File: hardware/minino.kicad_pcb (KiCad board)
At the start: 2 copper layers, 45 x 68 mm, 58 parts, among them J1 OLED, J2 GPS, J3 Battery, P1 USB_C_Plug_USB2.0, Q1 DMG3415U-7, Q2 MMBT2222A, SW1 ON, SW2 RIGHT, SW3 LEFT, SW4 DOWN, SW5 UP, SW6 OK, SW7 RESET, SW8 GPIO, U1 ESP32-S3-WROOM-1U-N16, U2 MCP73831-3-OT, U3 AP2112K-3.3

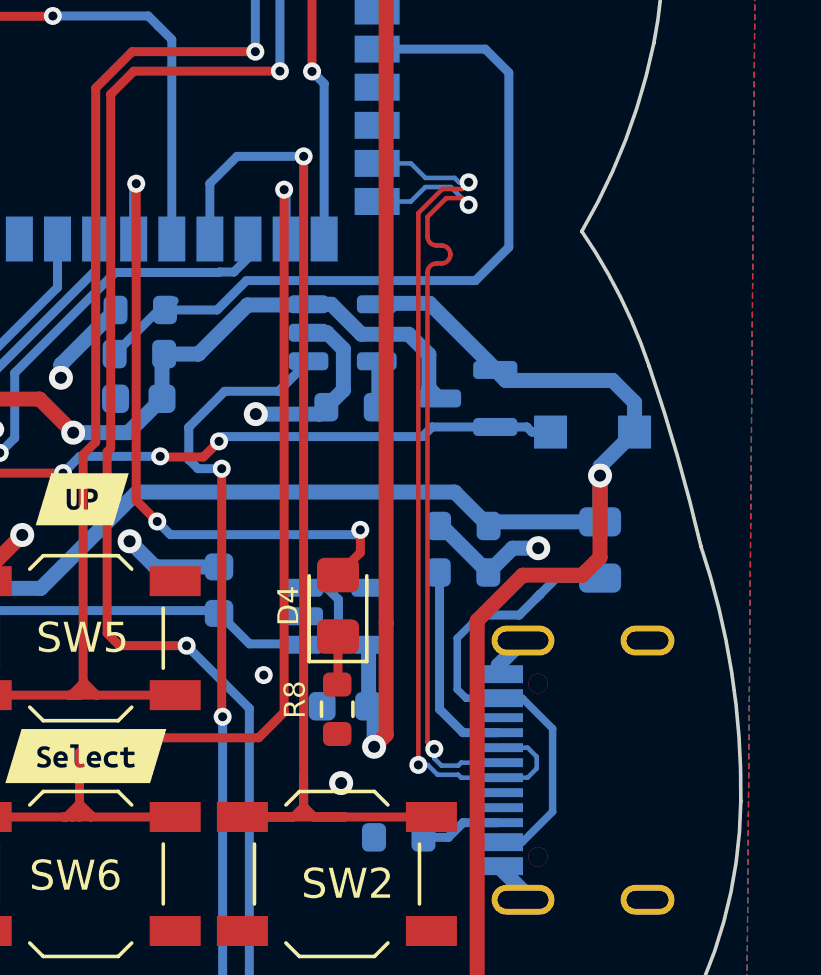
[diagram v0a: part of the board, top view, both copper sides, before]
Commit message: Add_example
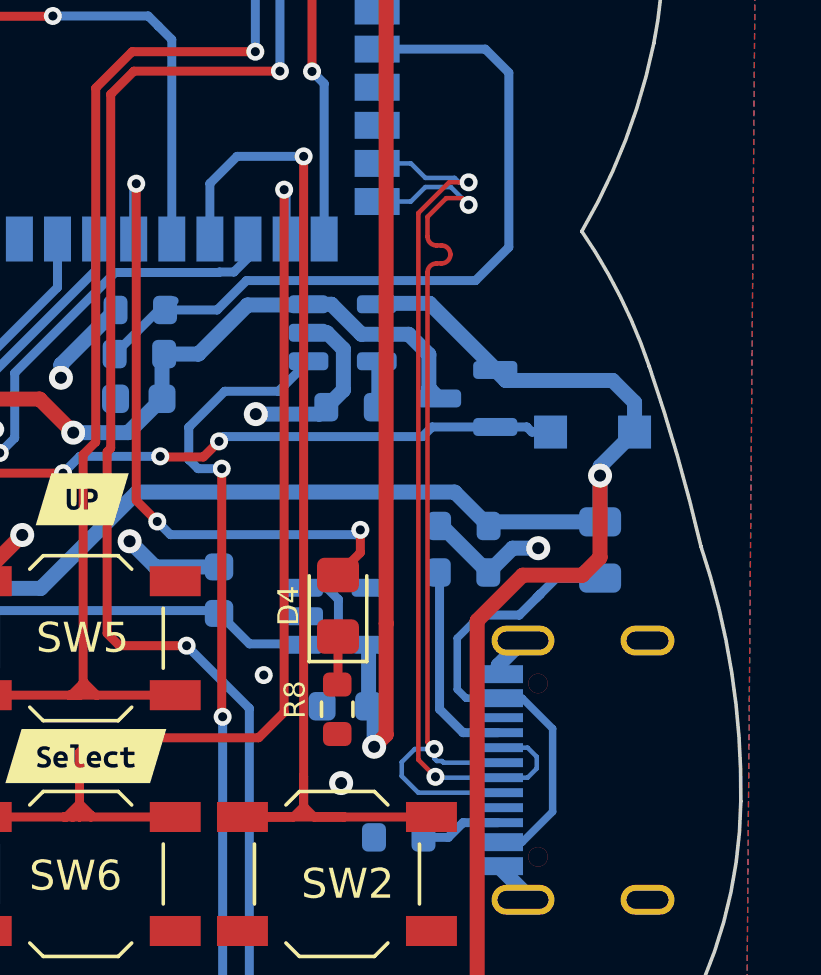
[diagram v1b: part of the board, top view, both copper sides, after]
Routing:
- net /D+: track 26.6 -> 31.7 mm
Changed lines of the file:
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@@
   (segment (start 198.585 76.82) (end 198.61 76.845) (width 0.3) (layer "B.Cu") (net 13))
   (segment (start 199.3925 82.16) (end 200.5675 82.16) (width 0.3) (layer "B.Cu") (net 13))
-  (segment (start 197.903986 64.840486) (end 198.706873 64.037599) (width 0.1524) (layer "F.Cu") (net 14))
-  (segment (start 197.903986 83.236014) (end 197.903986 64.840486) (width 0.1524) (layer "F.Cu") (net 14))
-  (segment (start 199.356201 64.037599) (end 199.58 63.8138) (width 0.1524) (layer "F.Cu") (net 14))
-  (segment (start 198.706873 64.037599) (end 199.356201 64.037599) (width 0.1524) (layer "F.Cu") (net 14))
+  (segment (start 198.930672 63.8138) (end 197.903986 64.840486) (width 0.1524) (layer "F.Cu") (net 14))
+  (segment (start 197.903986 83.062879) (end 198.473007 83.6319) (width 0.1524) (layer "F.Cu") (net 14))
+  (segment (start 199.58 63.8138) (end 198.930672 63.8138) (width 0.1524) (layer "F.Cu") (net 14))
+  (segment (start 197.903986 64.840486) (end 197.903986 83.062879) (width 0.1524) (layer "F.Cu") (net 14))
   (via (at 199.58 63.8138) (size 0.6) (drill 0.3) (layers "F.Cu" "B.Cu") (net 14))
-  (via (at 197.903986 83.236014) (size 0.6) (drill 0.3) (layers "F.Cu" "B.Cu") (net 14))
+  (via (at 198.473007 83.6319) (size 0.6) (drill 0.3) (layers "F.Cu" "B.Cu") (net 14))
   (segment (start 198.137601 63.6676) (end 197.655001 63.185) (width 0.1524) (layer "B.Cu") (net 14))
-  (segment (start 198.546873 83.5624) (end 198.220487 83.236014) (width 0.1524) (layer "B.Cu") (net 14))
-  (segment (start 199.232399 83.5624) (end 198.546873 83.5624) (width 0.1524) (layer "B.Cu") (net 14))
-  (segment (start 199.329999 83.66) (end 199.232399 83.5624) (width 0.1524) (layer "B.Cu") (net 14))
   (segment (start 201.85 83.3549) (end 201.85 82.9651) (width 0.1524) (layer "B.Cu") (net 14))
+  (segment (start 200.5675 83.66) (end 198.501107 83.66) (width 0.1524) (layer "B.Cu") (net 14))
+  (segment (start 198.501107 83.66) (end 198.473007 83.6319) (width 0.1524) (layer "B.Cu") (net 14))
   (segment (start 201.5449 82.66) (end 200.5675 82.66) (width 0.1524) (layer "B.Cu") (net 14))
   (segment (start 199.112453 63.6676) (end 198.137601 63.6676) (width 0.1524) (layer "B.Cu") (net 14))
@@
   (segment (start 201.85 82.9651) (end 201.5449 82.66) (width 0.1524) (layer "B.Cu") (net 14))
   (segment (start 200.5675 83.66) (end 201.5449 83.66) (width 0.1524) (layer "B.Cu") (net 14))
-  (segment (start 200.5675 83.66) (end 199.329999 83.66) (width 0.1524) (layer "B.Cu") (net 14))
   (segment (start 199.58 63.8138) (end 199.258653 63.8138) (width 0.1524) (layer "B.Cu") (net 14))
   (segment (start 201.5449 83.66) (end 201.85 83.3549) (width 0.1524) (layer "B.Cu") (net 14))
   (segment (start 197.655001 63.185) (end 196.53 63.185) (width 0.1524) (layer "B.Cu") (net 14))
-  (segment (start 198.220487 83.236014) (end 197.903986 83.236014) (width 0.1524) (layer "B.Cu") (net 14))
   (segment (start 198.833127 64.342401) (end 198.208786 64.966742) (width 0.1524) (layer "F.Cu") (net 15))
   (segment (start 198.208786 66.818786) (end 198.208786 66.868786) (width 0.1524) (layer "F.Cu") (net 15))
@@
   (arc (start 198.508786 66.518786) (mid 198.296654 66.606654) (end 198.208786 66.818786) (width 0.1524) (layer "F.Cu") (net 15))
   (arc (start 198.6713 65.918786) (mid 198.883432 66.006654) (end 198.9713 66.218786) (width 0.1524) (layer "F.Cu") (net 15))
+  (segment (start 197.35 83.61) (end 197.35 83.14) (width 0.1524) (layer "B.Cu") (net 15))
   (segment (start 197.655001 64.455) (end 196.53 64.455) (width 0.1524) (layer "B.Cu") (net 15))
-  (segment (start 199.232399 83.2576) (end 198.673127 83.2576) (width 0.1524) (layer "B.Cu") (net 15))
-  (segment (start 198.673127 83.2576) (end 198.436014 83.020487) (width 0.1524) (layer "B.Cu") (net 15))
-  (segment (start 199.329999 83.16) (end 199.232399 83.2576) (width 0.1524) (layer "B.Cu") (net 15))
-  (segment (start 200.5675 83.16) (end 199.329999 83.16) (width 0.1524) (layer "B.Cu") (net 15))
+  (segment (start 200.5675 83.16) (end 198.747264 83.16) (width 0.1524) (layer "B.Cu") (net 15))
+  (segment (start 198.691754 83.10449) (end 198.520017 83.10449) (width 0.1524) (layer "B.Cu") (net 15))
+  (segment (start 198.747264 83.16) (end 198.691754 83.10449) (width 0.1524) (layer "B.Cu") (net 15))
+  (segment (start 200.5675 84.16) (end 197.9 84.16) (width 0.1524) (layer "B.Cu") (net 15))
+  (segment (start 197.786014 82.703986) (end 198.436014 82.703986) (width 0.1524) (layer "B.Cu") (net 15))
+  (segment (start 197.35 83.14) (end 197.786014 82.703986) (width 0.1524) (layer "B.Cu") (net 15))
   (segment (start 198.9862 63.9724) (end 198.137601 63.9724) (width 0.1524) (layer "B.Cu") (net 15))
   (segment (start 199.58 64.5662) (end 198.9862 63.9724) (width 0.1524) (layer "B.Cu") (net 15))
   (segment (start 198.137601 63.9724) (end 197.655001 64.455) (width 0.1524) (layer "B.Cu") (net 15))
+  (segment (start 198.520017 83.10449) (end 198.436014 83.020487) (width 0.1524) (layer "B.Cu") (net 15))
   (segment (start 198.436014 83.020487) (end 198.436014 82.703986) (width 0.1524) (layer "B.Cu") (net 15))
+  (segment (start 197.9 84.16) (end 197.35 83.61) (width 0.1524) (layer "B.Cu") (net 15))
   (segment (start 199.3925 85.16) (end 198.9025 85.65) (width 0.3) (layer "B.Cu") (net 16))
   (segment (start 198.9025 85.65) (end 198.075 85.65) (width 0.3) (layer "B.Cu") (net 16))
